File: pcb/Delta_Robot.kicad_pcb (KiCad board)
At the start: 2 copper layers, 137 parts, among them J1 Conn_01x04, J2 USB_A, J3 USB_A, J4 Conn_01x02, J5 Conn_01x02, J6 MP3V5050VC6U, J7 RJ45, Q1 IRF9540STRLPBF, Q2 IRF9540STRLPBF, SW1 TL3305A, SW2 TL3305A, SW3 TL3305A, SW4 TL3305A, U1 LDL1117S33R, U2 LDL1117S33R, U3 ZLDO1117G12TA, U4 ICE40UP5K-SG48I, U5 W25Q64JVSSIQ, U6 STM32F412RGT6, U7 Omega2+, U8 4N25-X007T, U9 4N25-X007T, Y1 Crystal

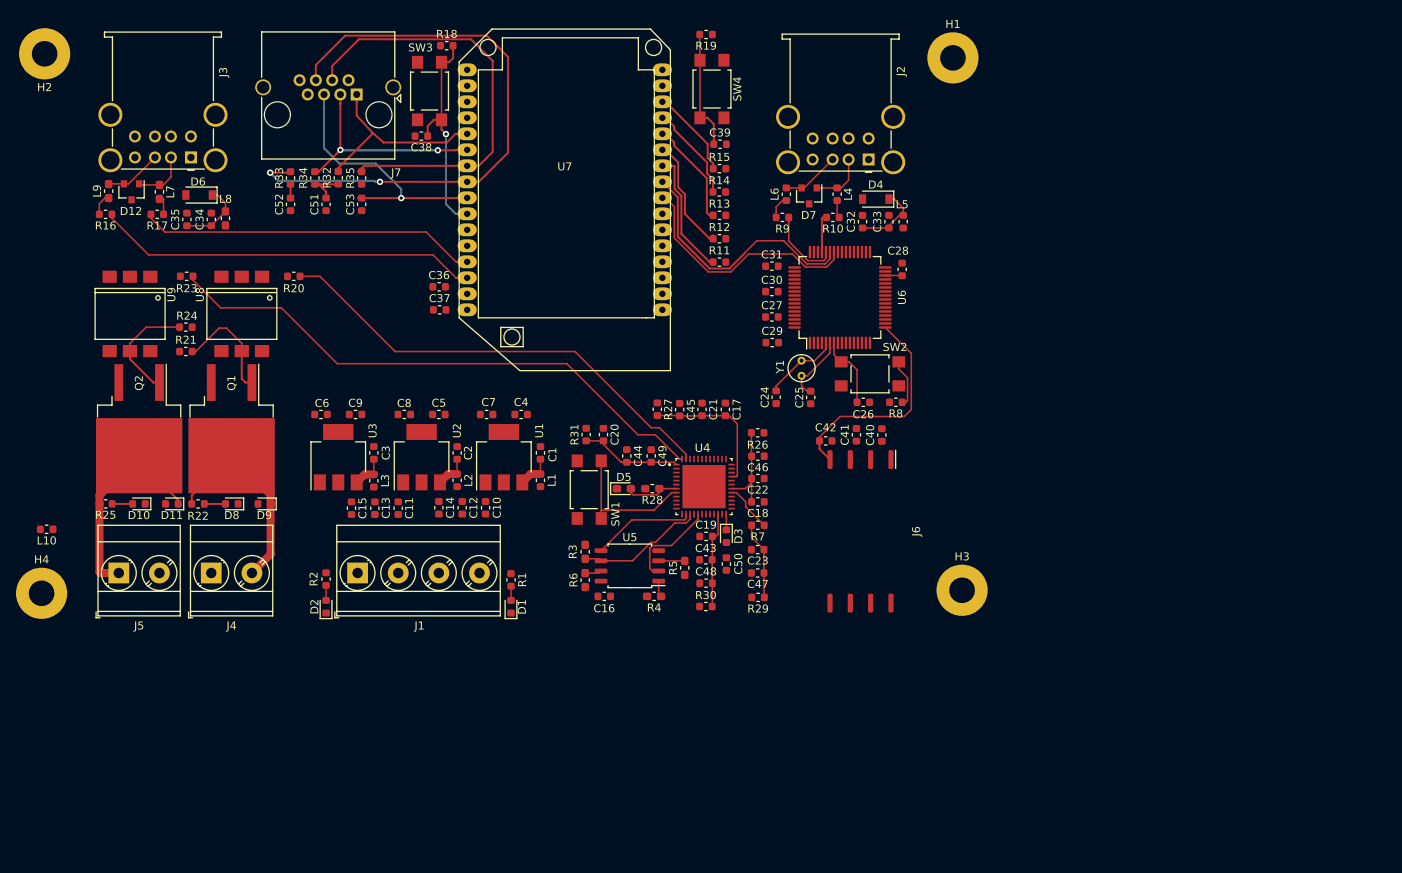
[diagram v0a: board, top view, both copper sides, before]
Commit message: Modificacion general PCB
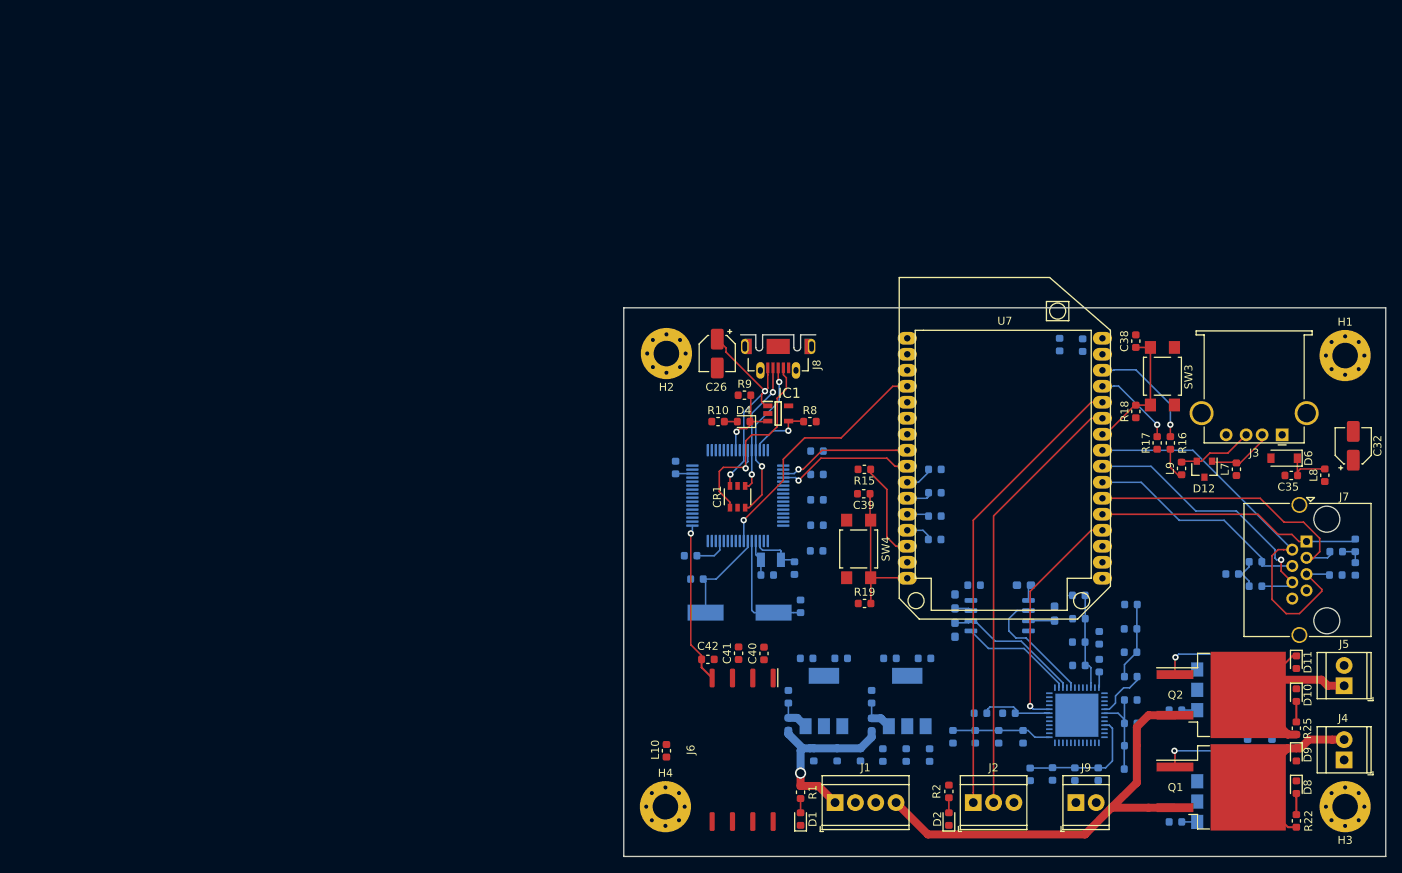
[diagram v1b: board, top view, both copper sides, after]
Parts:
- removed C1: 1uF, Capacitor_SMD:C_0603_1608Metric
- removed C33, C4: 0.1uF, Capacitor_SMD:C_0603_1608Metric
- removed C7: 4.7uF, Capacitor_SMD:C_0603_1608Metric
- removed D7: NUP2105L, Package_TO_SOT_SMD:SOT-23
- removed L1: BLM18SG121TN1D, Inductor_SMD:L_0603_1608Metric
- removed L4, L6: SRF2012-900YA, Inductor_SMD:L_0603_1608Metric
- removed L5: 742792651, Inductor_SMD:L_0603_1608Metric
- removed SW1, SW2: TL3305A, Button_Switch_SMD:SW_SPST_TL3305A
- removed U1: LDL1117S33R, Package_TO_SOT_SMD:SOT-223-3_TabPin2
- added C54: 2pF, Capacitor_SMD:C_0603_1608Metric, B.Cu at (108.1, 90.6)
- added C55: 0.1uF, Capacitor_SMD:C_0603_1608Metric, B.Cu at (114.3, 75.1)
- added CR1: ESDA6V1BC6, SMD:ESDA6V1BC6, F.Cu at (104.4, 80.8)
- added IC1: STMPS2151STR, SMD:SOT95P280X145-5N, F.Cu at (109.5, 70.4)
- added J8: 47590-0001, SMD:MOLEX_47590-0001, F.Cu at (109.5, 62.0)
- added J9: Conn_01x02, TerminalBlock_TE-Connectivity:TerminalBlock_TE_282834-2_1x02_P2.54mm_Horizontal, F.Cu at (146.7, 119.0)
- added L11: SRF2012-900YA, Inductor_SMD:L_0603_1608Metric, B.Cu at (98.5, 88.1)
- added Y2: 32.768KHZ, Crystal:Crystal_SMD_3215-2Pin_3.2x1.5mm, B.Cu at (108.6, 88.6)
- C10, C11, C12, C13, C14, C15, C16, C17, C18, C19, C2, C20, C21, C22, C23, C27, C28, C29, C3, C30, C31, C36, C37, C43, C44, C45, C46, C47, C48, C49, C5, C50, C51, C52, C53, C6, C8, C9, D3, L2, L3, R11, R12, R13, R14, R21, R24, R26, R27, R29, R3, R30, R31, R32, R33, R34, R35, R4, R5, R6, R7, U2, U3, U4, U5, U6, U8, U9: moved to B.Cu
- C24, C25: value 0.1uF -> 4.3pF; moved to B.Cu
- C26: value 0.1uF -> 4.7uF; footprint Capacitor_SMD:C_0603_1608Metric -> Capacitor_SMD:CP_Elec_4x3
- C32: footprint Capacitor_SMD:C_0603_1608Metric -> Capacitor_SMD:CP_Elec_4x3
- C34: value 22u -> 2pF; moved to B.Cu
- D4: value 1N4733AW -> LED; footprint Diode_SMD:D_SOD-123 -> LED_SMD:LED_0603_1608Metric
- D5: footprint LED_SMD:LED_0603_1608Metric_Pad1.05x0.95mm_HandSolder -> LED_SMD:LED_0603_1608Metric; moved to B.Cu
- H1, H2, H3, H4: footprint MountingHole:MountingHole_3.2mm_M3_Pad -> MountingHole:MountingHole_3.2mm_M3_Pad_Via
- J1: footprint TerminalBlock_Phoenix:TerminalBlock_Phoenix_MKDS-3-4-5.08_1x04_P5.08mm_Horizontal -> TerminalBlock_TE-Connectivity:TerminalBlock_TE_282834-4_1x04_P2.54mm_Horizontal
- J2: value USB_A -> Conn_01x03; footprint Connector_USB:USB_A_Wuerth_61400826021_Horizontal_Stacked -> TerminalBlock_TE-Connectivity:TerminalBlock_TE_282834-3_1x03_P2.54mm_Horizontal
- J3: footprint Connector_USB:USB_A_Wuerth_61400826021_Horizontal_Stacked -> Connector_USB:USB_A_Stewart_SS-52100-001_Horizontal
- J4, J5: footprint TerminalBlock_Phoenix:TerminalBlock_Phoenix_MKDS-3-2-5.08_1x02_P5.08mm_Horizontal -> TerminalBlock_TE-Connectivity:TerminalBlock_TE_282834-2_1x02_P2.54mm_Horizontal
- L7, L8, L9: footprint Inductor_SMD:L_0603_1608Metric_Pad1.05x0.95mm_HandSolder -> Inductor_SMD:L_0603_1608Metric
- R10: value 0K -> 620
- R20, R23: value 100 -> 330; moved to B.Cu
- R28: footprint Resistor_SMD:R_0603_1608Metric_Pad1.05x0.95mm_HandSolder -> Resistor_SMD:R_0603_1608Metric; moved to B.Cu
- R9: value 0K -> 10k
- Y1: value Crystal -> 8MHz; footprint Crystal:Crystal_C38-LF_D3.0mm_L8.0mm_Vertical -> Crystal:Crystal_SMD_HC49-SD; moved to B.Cu
- moved J5 153.8 mm to (180.2, 104.4), turned to 90 degrees
- moved R25 151.4 mm to (174.2, 109.7), turned to 90 degrees
- moved D10 146.6 mm to (174.2, 105.6), turned to 270 degrees
- moved U9 145.8 mm to (166.5, 104.9), turned to 90 degrees
- moved R21 144.4 mm to (171.2, 111.9), turned to 270 degrees
- moved J4 143.5 mm to (180.2, 113.7), turned to 90 degrees
- moved R22 142.9 mm to (174.2, 121.3), turned to 90 degrees
- moved R24 142.7 mm to (168.1, 111.9), turned to 90 degrees
- moved D11 141.9 mm to (174.2, 101.4), turned to 270 degrees
- moved C35 141.7 mm to (173.6, 78.1), turned to 180 degrees
- moved L8 141.1 mm to (177.8, 78.1)
- moved J3 140.7 mm to (172.5, 73.0)
- moved D6 139.6 mm to (172.7, 75.9)
- moved Q2 139.3 mm to (164.8, 105.5), turned to 0 degrees
- moved L7 139.0 mm to (166.8, 77.3)
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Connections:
- C16 pad 1: +3V3_FPGA -> +3V3
- C26 pad 1: Net-(C26-Pad1) -> /STM32/STM32_USB_VBUS
- C27 pad 1: +3.3V_ESP32 -> +3V3
- C29 pad 1: +3.3V_ESP32 -> +3V3
- C30 pad 1: +3.3V_ESP32 -> +3V3
- C31 pad 1: +3.3V_ESP32 -> +3V3
- C35 pad 1: Net-(C34-Pad1) -> Net-(C32-Pad1)
- C36 pad 1: +3V3_OMEGA2+ -> +3V3
- C37 pad 1: +3V3_OMEGA2+ -> +3V3
- C40 pad 1: +3.3V_ESP32 -> +3V3
- C41 pad 1: +3.3V_ESP32 -> +3V3
- C5 pad 1: +3V3_FPGA -> +3V3
- C50 pad 1: +3V3_FPGA -> +3V3
- C8 pad 1: +3V3_FPGA -> +3V3
- D3 pad 2: +3V3_FPGA -> +3V3
- D4 pad 1: Net-(C32-Pad1) -> /STM32/STM32_USB_OverCurrent
- D4 pad 2: GND -> Net-(D4-Pad2)
- D6 pad 1: Net-(C34-Pad1) -> Net-(C32-Pad1)
- J1 pad 1: +24V -> +5V
- J1 pad 2: GNDPWR -> GND
- J1 pad 3: GND -> GNDPWR
- J1 pad 4: +5V -> +24V
- J2 pad 1: GND -> /External Communications/EXT_RS232_TX
- J2 pad 2: Net-(D7-Pad1) -> /External Communications/EXT_RS232_RX
- J2 pad 3: Net-(D7-Pad2) -> GND
- J6 pad 2: +3.3V_ESP32 -> +3V3
- L8 pad 1: (no net) -> +5V
- L8 pad 2: Net-(C34-Pad1) -> Net-(C32-Pad1)
- R10 pad 1: Net-(L4-Pad1) -> Net-(D4-Pad2)
- R10 pad 2: /STM32/STM32_USB_D- -> +3V3
- R18 pad 1: +3V3_OMEGA2+ -> +3V3
- R19 pad 1: +3V3_OMEGA2+ -> +3V3
- R27 pad 2: +3V3_FPGA -> +3V3
- R28 pad 2: +3V3_FPGA -> +3V3
- R3 pad 1: +3V3_FPGA -> +3V3
- R30 pad 2: +3V3_FPGA -> +3V3
- R31 pad 2: +3V3_FPGA -> +3V3
- R5 pad 1: +3V3_FPGA -> +3V3
- R6 pad 1: +3V3_FPGA -> +3V3
- R8 pad 1: Net-(C26-Pad1) -> GND
- R8 pad 2: +3.3V_ESP32 -> /STM32/STM32_USB_PowerSwitchOn
- R9 pad 1: /STM32/STM32_USB_D+ -> /STM32/STM32_USB_OverCurrent
- R9 pad 2: Net-(L6-Pad1) -> +3V3
- U2 pad 2: +3V3_FPGA -> +3V3
- U4 pad 25: (no net) -> /FPGA/FPGA_SOLENOID1
- U4 pad 26: (no net) -> /FPGA/FPGA_SOLENOID2
- U4 pad 47: /FPGA/FPGA_SOLENOID1 -> (no net)
- U4 pad 48: /FPGA/FPGA_SOLENOID2 -> (no net)
- U4 pad 8: /FPGA/FPGA_CRESET_B -> /FPGA/~FPGA_CRESET_B
- U5 pad 8: +3V3_FPGA -> +3V3
- U6 pad 13: (no net) -> Net-(L11-Pad2)
- U6 pad 19: +3.3V_ESP32 -> +3V3
- U6 pad 3: (no net) -> Net-(C34-Pad1)
- U6 pad 32: +3.3V_ESP32 -> +3V3
- U6 pad 4: (no net) -> Net-(C54-Pad1)
- U6 pad 40: (no net) -> /STM32/STM32_USB_OverCurrent
- U6 pad 42: /Onion Omega 2/ONION_SER1_RX -> /STM32/STM32_USB_VBUS
- U6 pad 43: /Onion Omega 2/ONION_SER1_TX -> /STM32/STM32_USB_ID
- U6 pad 44: /STM32/STM32_USB_D+ -> /STM32/STM32_USB_DM
- U6 pad 45: /STM32/STM32_USB_D- -> /STM32/STM32_USB_DP
- U6 pad 46: (no net) -> /STM32/STM32_USB_PowerSwitchOn
- U6 pad 48: +3.3V_ESP32 -> +3V3
- U6 pad 51: (no net) -> /Onion Omega 2/ONION_SER1_RX
- U6 pad 52: (no net) -> /Onion Omega 2/ONION_SER1_TX
- U6 pad 64: +3.3V_ESP32 -> +3V3
- U6 pad 7: Net-(C26-Pad1) -> /Onion Omega 2/STM32_NRST
- U7 pad 20: (no net) -> /FPGA/~FPGA_CRESET_B
- U7 pad 27: (no net) -> /External Communications/EXT_RS232_RX
- U7 pad 28: (no net) -> /External Communications/EXT_RS232_TX
- U7 pad 31: +3V3_OMEGA2+ -> +3V3
- U7 pad 4: (no net) -> /Onion Omega 2/STM32_NRST
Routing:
- net /FPGA/FPGA_SOLENOID2: track 70.9 -> 0.00 mm
- net /FPGA/FPGA_SOLENOID1: track 58.1 -> 0.00 mm
- net /External Communications/EXT_RS232_TX: track 0.00 -> 57.5 mm
- net +24V: track 0.00 -> 54.7 mm
- net /External Communications/EXT_RS232_RX: track 0.00 -> 54.5 mm
- net /Onion Omega 2/OMEGA2_ETH_TX-: track 74.8 -> 35.2 mm, vias 2 -> 1
- net /Onion Omega 2/OMEGA2_USB_D+: track 49.4 -> 14.3 mm, vias 0 -> 1
- net /Onion Omega 2/OMEGA2_USB_D-: track 42.3 -> 10.4 mm, vias 0 -> 1
- net /Onion Omega 2/STM32_NRST: track 0.00 -> 31.6 mm, vias 0 -> 1
- net /FPGA/~FPGA_CRESET_B: track 0.00 -> 29.1 mm, vias 0 -> 1
- net /STM32/STM32_USB_VBUS: track 0.00 -> 28.2 mm, vias 0 -> 2
- net /STM32/STM32_USB_ID: track 0.00 -> 27.1 mm, vias 0 -> 1
- net /Onion Omega 2/OMEGA2_ETH_TX+: track 53.9 -> 28.6 mm
- net +5V: track 0.00 -> 23.9 mm, vias 0 -> 1
- net /STM32/STM32_USB_DP: track 0.00 -> 20.2 mm, vias 0 -> 2
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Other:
- board outline added: 95.2 x 68.6 mm
